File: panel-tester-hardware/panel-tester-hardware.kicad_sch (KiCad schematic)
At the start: 21 parts, among them J1 Screw_Terminal_01x02, J2 Conn_01x02, J3 Conn_01x07, Q2 BS170, U3 LM358, U4 INA219AxD

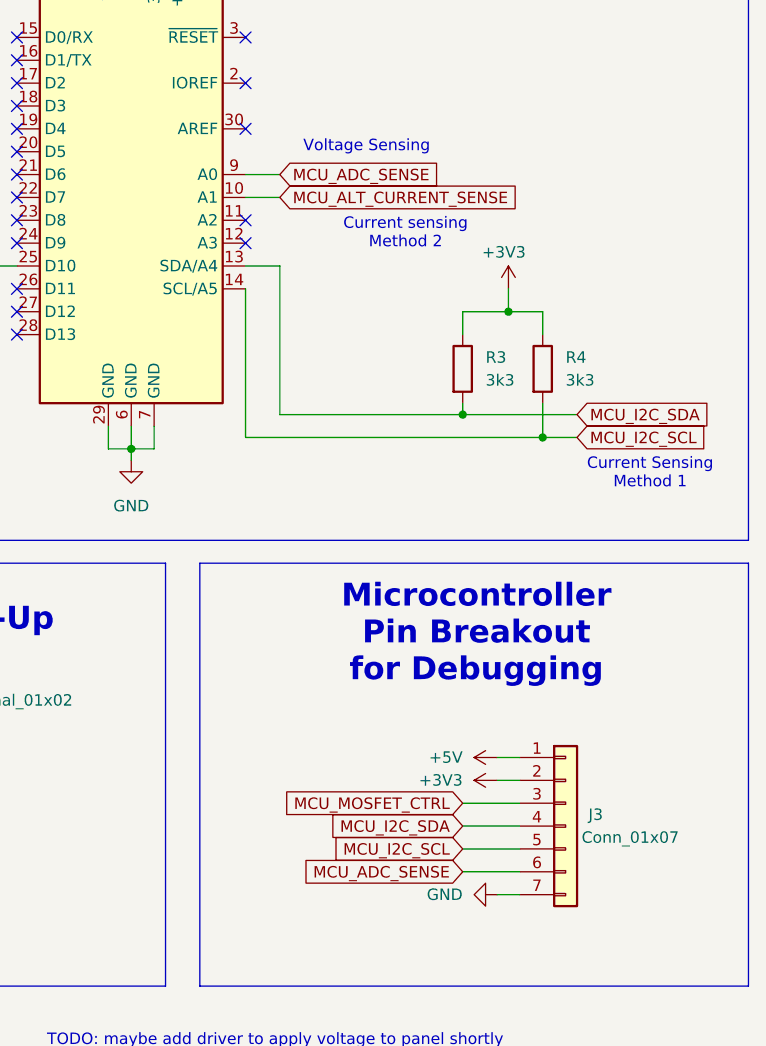
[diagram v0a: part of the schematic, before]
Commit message: Did a lot of things
Created board layout and completed routing
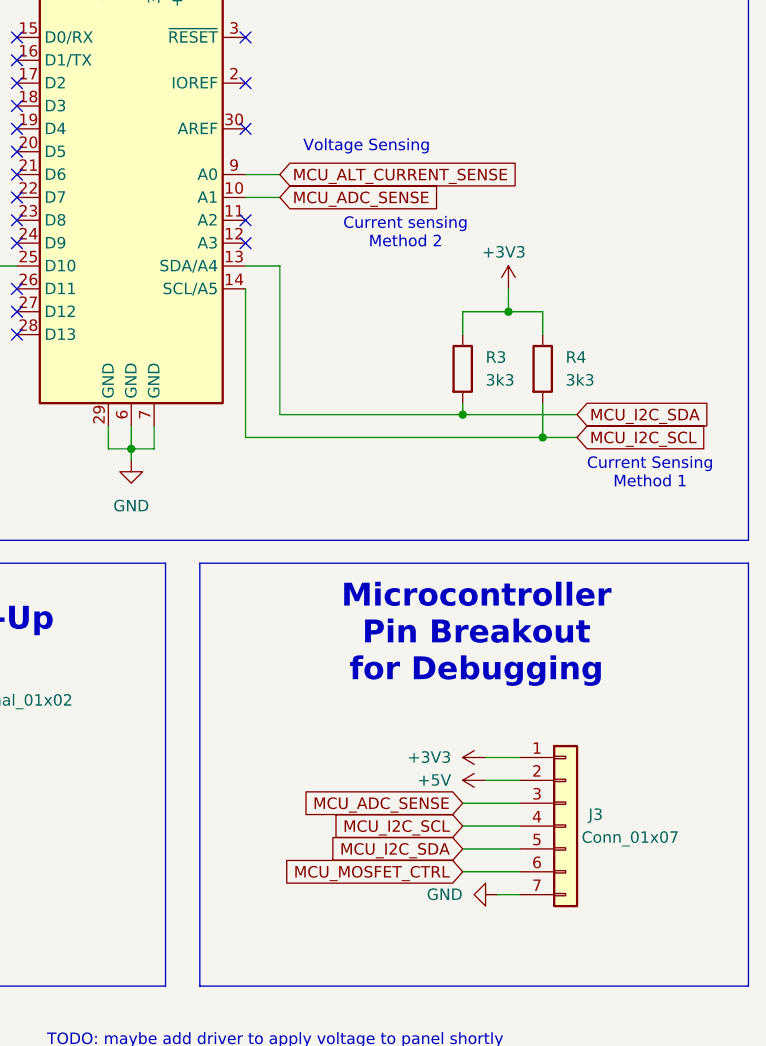
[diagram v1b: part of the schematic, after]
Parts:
- Q2: footprint Package_TO_SOT_THT:TO-92_Inline -> Package_TO_SOT_THT:TO-220-3_Vertical
- U3: footprint Package_SO:SOIC-8_3.9x4.9mm_P1.27mm -> Package_DIP:DIP-8_W7.62mm_LongPads
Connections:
- net +3V3: now also J3.1 (Pin_1); no longer J3.2 (Pin_2)
- net +5V: now also J3.2 (Pin_2); no longer J3.1 (Pin_1)
- net MCU_ADC_SENSE: now also A1.10 (A1), J3.3 (Pin_3); no longer A1.9 (A0), J3.6 (Pin_6)
- net MCU_ALT_CURRENT_SENSE: now also A1.9 (A0); no longer A1.10 (A1)
- net MCU_I2C_SCL: now also J3.4 (Pin_4); no longer J3.5 (Pin_5)
- net MCU_I2C_SDA: now also J3.5 (Pin_5); no longer J3.4 (Pin_4)
- net MCU_MOSFET_CTRL: now also J3.6 (Pin_6); no longer J3.3 (Pin_3)
